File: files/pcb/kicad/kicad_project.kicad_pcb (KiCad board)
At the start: 2 copper layers, 100 x 91.5 mm, 107 parts, among them CON1 USB_MINI_B, IC1 ATMEGA328-A, IC10 MY_FET_P, IC11 DS1307, IC12 MY_NPN, IC13 MY_PNP, IC14 MY_FET_N, IC2 74LC138, IC3 TLP627, IC4 TLP627, IC5 SN74141_K155NA, IC6 TLP627-4, IC7 TLP627-4, IC8 MY_3_TERMINAL_REGULATOR, IC9 ICM7555CD, K1 CONN_3, K2 CONN_3, K3 CONN_3, K4 CONN_3, P1 CONN_6, SW3 SW_PUSH, SW4 SW_PUSH, SW5 SW_PUSH, T1 2SC, U1 NEON, U10 NIXIE_IN_16, U11 DC_JACK, U15 MY_PIN52, U16 MY_PIN52, U17 MY_PIN52, U18 MY_PIN52, U2 NEON, U3 NEON, U4 NEON, U5 NIXIE_IN_16, U6 NIXIE_IN_16, U7 NIXIE_IN_16, U8 NIXIE_IN_16, U9 NIXIE_IN_16, X1 12MHz, X2 32.768kHz

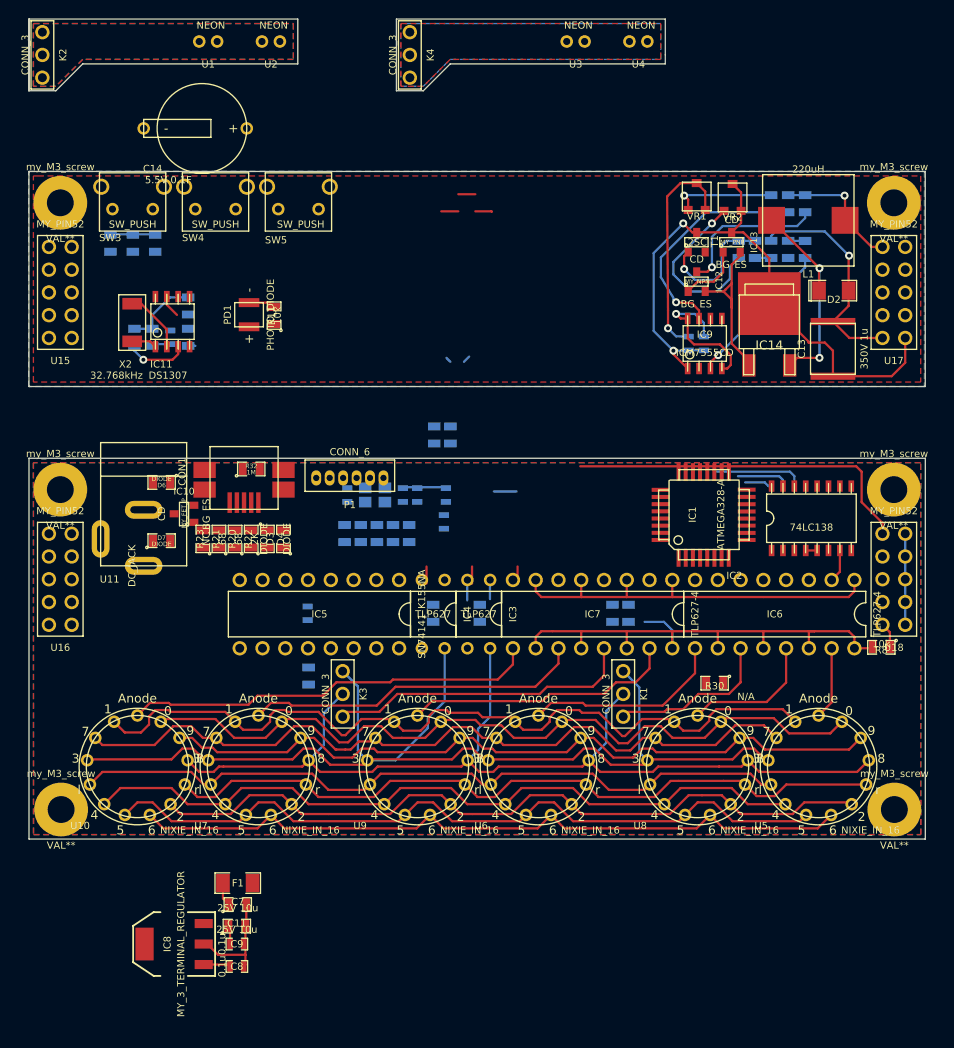
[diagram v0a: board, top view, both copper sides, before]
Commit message: PCB更新
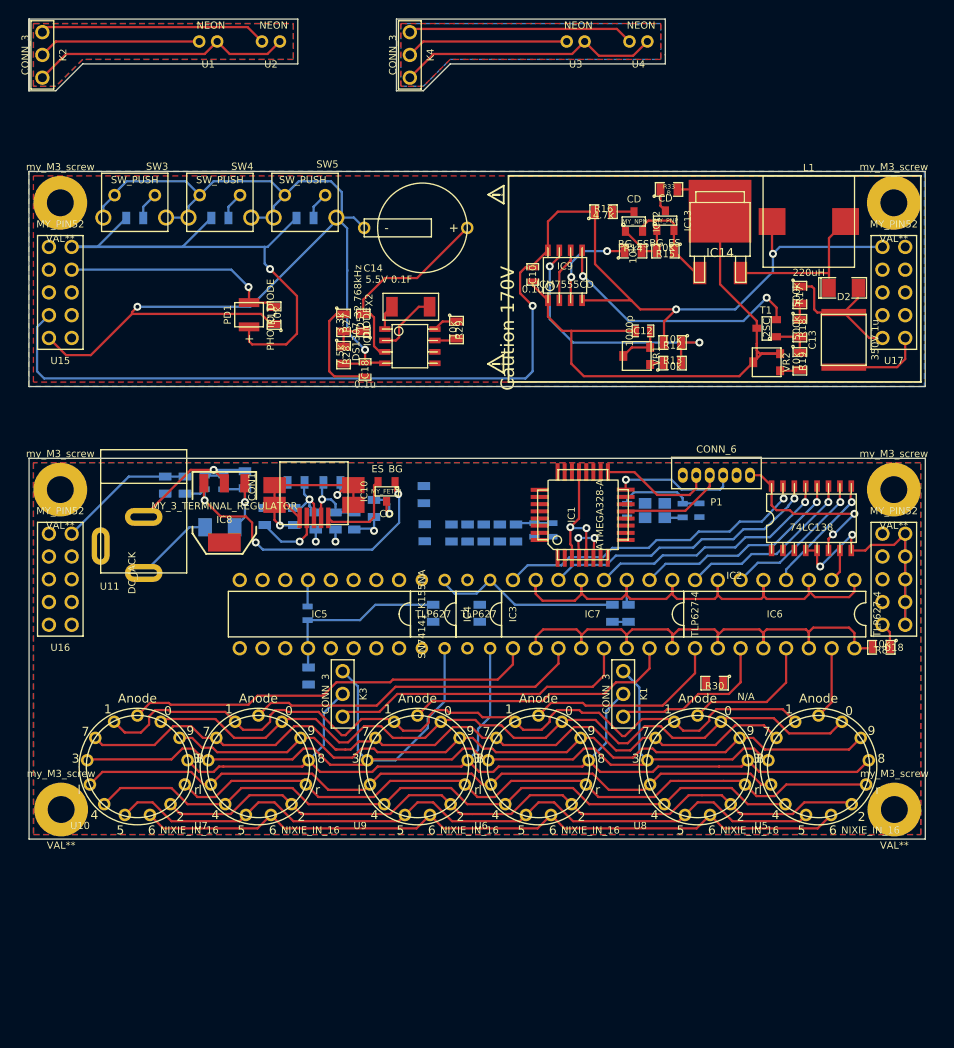
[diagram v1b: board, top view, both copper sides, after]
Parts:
- added R33: R, SM0805, F.Cu at (167.1, 68.3)
- C10, C12, C18, D5, R12, R13, R14, R15, R16, R17, R18, R19, R27, R28, R29: moved to F.Cu
- C11, C7, C8, C9, D3, D4, D6, D7, F1, R20, R21, R22, R23, R32: moved to B.Cu
- moved C8 54.0 mm to (117.4, 101.0), turned to 90 degrees
- moved C9 51.6 mm to (115.3, 101.0), turned to 90 degrees
- moved C11 49.8 mm to (110.9, 101.3), turned to 270 degrees
- moved IC8 48.4 mm to (117.5, 104.4), turned to 180 degrees
- moved C7 47.4 mm to (119.8, 100.7), turned to 90 degrees
- moved P1 40.9 mm to (172.4, 100.2)
- moved F1 39.8 mm to (117.0, 106.0), turned to 0 degrees
- moved X2 33.2 mm to (140.4, 81.4), turned to 180 degrees
- moved C1 31.5 mm to (170.5, 104.1)
- moved C4 31.3 mm to (168.6, 104.1)
- moved C5 31.3 mm to (162.4, 104.1)
- moved X1 31.3 mm to (166.6, 104.9)
- moved R29 29.9 mm to (143.4, 84.0)
- moved C14 27.0 mm to (139.6, 72.6)
- moved IC11 26.6 mm to (138.2, 85.8), turned to 270 degrees
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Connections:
- IC13 pad 3: PINGND -> N-0000098
- U15 pad 10: PIN5V -> PINADC6
- U15 pad 4: (no net) -> PIN9V
- U15 pad 6: PINSCL -> PIN5V
- U15 pad 7: PINSDA -> PINSCL
- U15 pad 8: PINCLKOUT -> PINSDA
- U15 pad 9: PINADC6 -> PINCLKOUT
- U16 pad 10: +5V -> /ADC6
- U16 pad 4: (no net) -> +9V
- U16 pad 6: /SCL -> +5V
- U16 pad 7: /SDA -> /SCL
- U16 pad 8: /PD4 -> /SDA
- U16 pad 9: /ADC6 -> /PD4
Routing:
- net PINGND: track 71.0 -> 209.4 mm
- net PIN9V: track 31.1 -> 145.0 mm, vias 2 -> 3
- net GND: track 28.4 -> 141.5 mm, vias 0 -> 7
- net +5V: track 2.08 -> 45.3 mm, vias 0 -> 5
- net PIN5V: track 5.05 -> 47.3 mm, vias 0 -> 1
- net PINADC6: track 3.01 -> 44.3 mm, vias 0 -> 1
- net N-0000089: track 0.00 -> 36.6 mm, vias 0 -> 3
- net /nixie/L8: track 1.91 -> 35.5 mm, vias 0 -> 1
- net /nixie/L7: track 0.00 -> 31.5 mm, vias 0 -> 1
- net +9V: track 39.5 -> 8.96 mm
- net N-0000090: track 0.00 -> 29.6 mm, vias 0 -> 2
- net N-00000107: track 0.00 -> 29.5 mm
- net N-00000110: track 0.00 -> 29.3 mm
- net (no net): track 28.7 -> 0.00 mm
- net /nixie/L6: track 0.00 -> 27.8 mm, vias 0 -> 1
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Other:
- board text added: "Caution 170V"
